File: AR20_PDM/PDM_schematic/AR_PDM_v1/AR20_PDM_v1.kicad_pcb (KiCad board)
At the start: 2 copper layers, 118 x 112 mm, 253 parts, among them IC1 TMUX1208PWR, J1 S_T_?, J2 1-776163-1, K1 DIPxx-1Cxx-51x, K2 DIPxx-1Cxx-51x, P1 B4B-PH-SM4-TB, Q1 BTS50025-1TAD, Q2 BTS50025-1TAD, Q3 BTS50025-1TAD, Q5 BTS50025-1TAD, Q6 BTS50025-1TAD, Q7 BTS50025-1TAD, Q8 BTS50025-1TAD, SW1 SW_DIP_x07, U1 ACM_2020, U10 N-MOS, U11 N-MOS, U12 P-MOS, U13 N-MOS, U14 N-MOS, U15 NMOS, U16 NMOS, U17 NMOS, U18 NMOS, U19 NMOS, U2 INA233, U20 NMOS, U21 NMOS, U22 NMOS, U23 NMOS, U24 NMOS, U25 NMOS, U26 NMOS, U27 NMOS, U28 NMOS, U29 INA233, U3 INA233, U30 INA233, U31 INA233, U32 Fet-P, U33 Fet-P, U34 Fet-P, U35 Fet-P, U36 Fet-P, U4 INA233, U5 INA233, U6 INA233, U7 INA233, U8 INA233, U9 TCA6424ARGJR

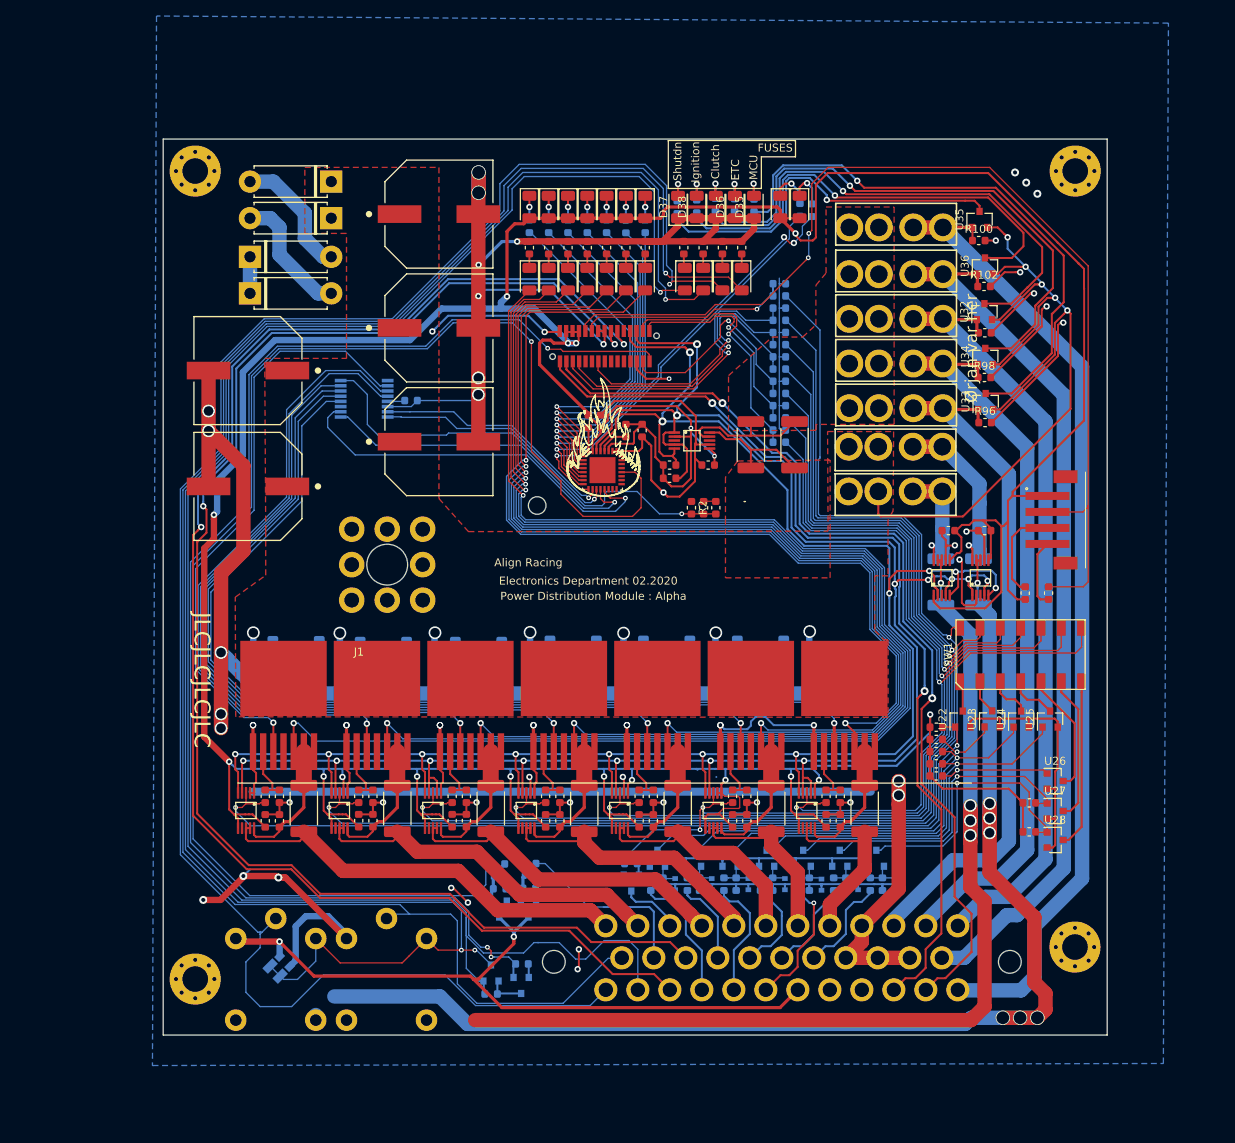
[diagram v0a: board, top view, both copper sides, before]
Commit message: Pdm version B Draft finished
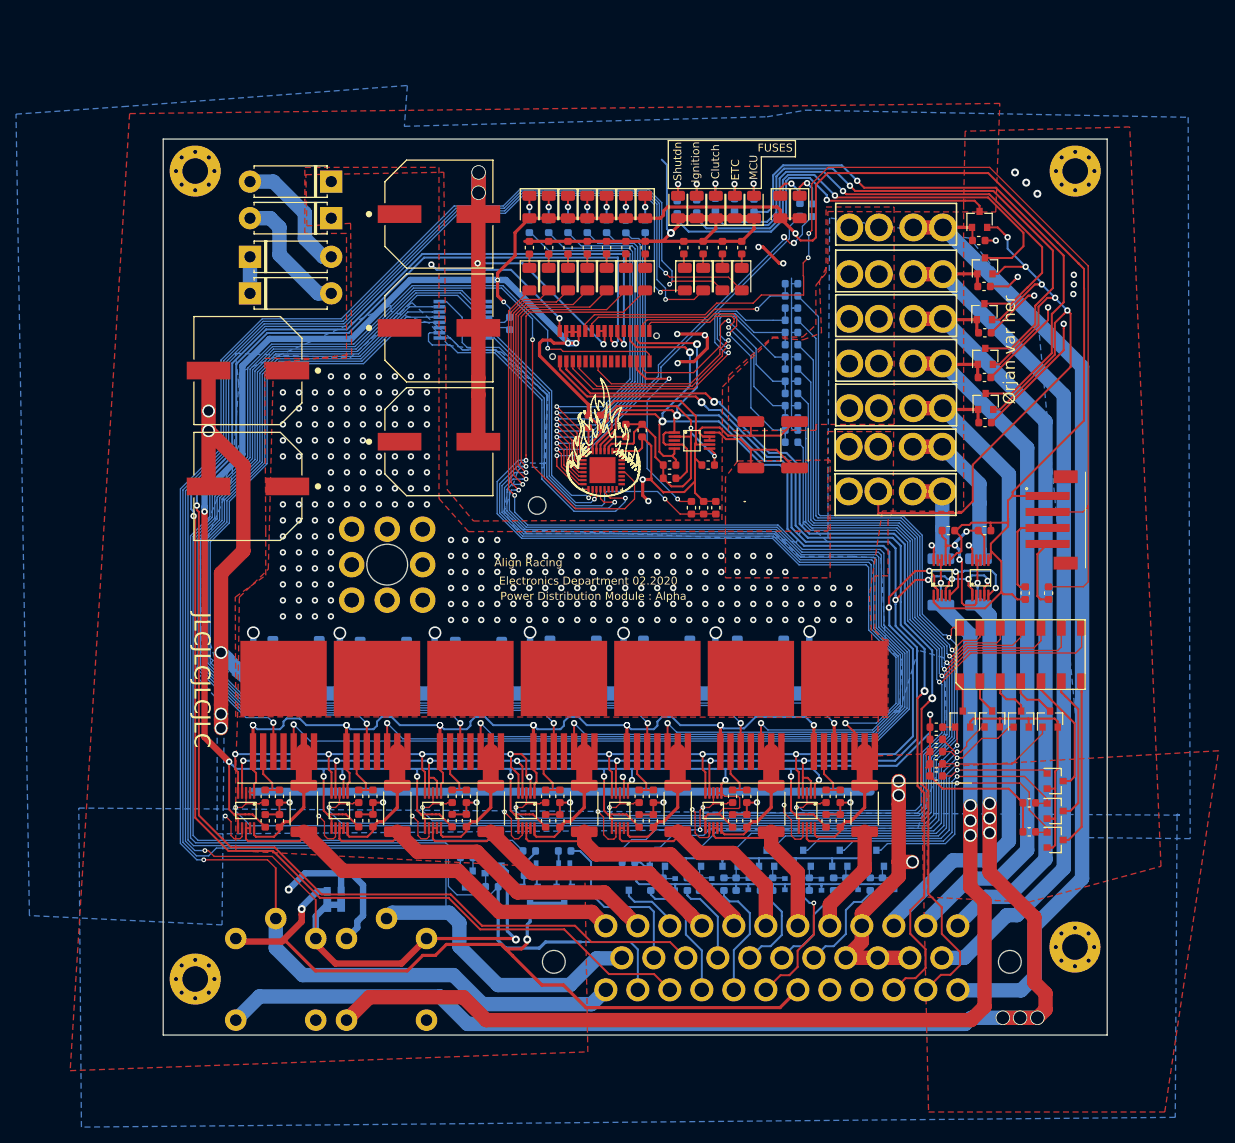
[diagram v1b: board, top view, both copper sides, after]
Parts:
- moved IC1 15.8 mm to (71.3, 58.9)
- moved C47 15.7 mm to (77.2, 59.4), turned to 270 degrees
- moved U11 15.0 mm to (71.6, 128.8)
- moved R89 15.0 mm to (71.8, 126.1)
- moved U12 13.4 mm to (75.1, 127.2), turned to 0 degrees
- moved R5 13.4 mm to (74.9, 129.8), turned to 0 degrees
- moved D30 11.6 mm to (56.1, 131.4), turned to 90 degrees
- moved D31 10.3 mm to (54.4, 131.4), turned to 90 degrees
- moved U14 4.79 mm to (84.0, 130.9)
- moved R92 4.66 mm to (84.0, 128.4)
- moved R105 4.64 mm to (84.0, 125.3)
- moved D40 4.61 mm to (84.0, 126.8)
- moved D39 4.30 mm to (79.8, 126.8)
- moved U13 4.23 mm to (79.7, 130.9)
- moved R90 4.21 mm to (79.8, 128.4)
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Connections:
- IC1 pad 3: (no net) -> Net-(IC1-Pad3)
- IC1 pad 9: (no net) -> Net-(IC1-Pad9)
- J2 pad 31: (no net) -> Net-(J2-Pad31)
- J2 pad 32: (no net) -> Net-(J2-Pad32)
- K1 pad 1: (no net) -> Net-(K1-Pad1)
- K2 pad 1: (no net) -> Net-(K2-Pad1)
- Q1 pad 4: (no net) -> Net-(Q1-Pad4)
- Q2 pad 4: (no net) -> Net-(Q2-Pad4)
- Q3 pad 4: (no net) -> Net-(Q3-Pad4)
- Q5 pad 4: (no net) -> Net-(Q5-Pad4)
- Q6 pad 4: (no net) -> Net-(Q6-Pad4)
- Q7 pad 4: (no net) -> Net-(Q7-Pad4)
- Q8 pad 4: (no net) -> Net-(Q8-Pad4)
- SW1 pad 12: (no net) -> P3_MOS_IN
- U1 pad 10: (no net) -> Net-(U1-Pad10)
- U1 pad 11: (no net) -> Net-(U1-Pad11)
- U1 pad 13: (no net) -> Net-(U1-Pad13)
- U1 pad 15: (no net) -> Net-(U1-Pad15)
- U1 pad 19: (no net) -> Net-(U1-Pad19)
- U1 pad 21: (no net) -> Net-(U1-Pad21)
- U1 pad 7: (no net) -> Net-(U1-Pad7)
- U1 pad 9: (no net) -> Net-(U1-Pad9)
- U29 pad 3: (no net) -> /Fuel_Ignition_ShutdownCircuit/COIL_INJECTOR_Alert
- U30 pad 3: (no net) -> /Fuel_Ignition_ShutdownCircuit/FP_Alert
- U31 pad 3: (no net) -> /Fuses_Direct/DIRECT_Alert
- U9 pad 14: (no net) -> Net-(U9-Pad14)
- U9 pad 15: (no net) -> Net-(U9-Pad15)
- U9 pad 16: (no net) -> Net-(U9-Pad16)
- U9 pad 17: (no net) -> Net-(U9-Pad17)
- U9 pad 18: (no net) -> Net-(U9-Pad18)
- U9 pad 19: (no net) -> Net-(U9-Pad19)
- U9 pad 21: (no net) -> Net-(U9-Pad21)
- U9 pad 22: (no net) -> Net-(U9-Pad22)
- U9 pad 23: (no net) -> Net-(U9-Pad23)
- U9 pad 24: (no net) -> Net-(U9-Pad24)
- U9 pad 33: (no net) -> Net-(U9-Pad33)
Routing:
- net GND: track 842.3 -> 961.9 mm, vias 56 -> 64
- net P7_MOS_SENSE: track 125.2 -> 147.7 mm
- net P6_MOS_SENSE: track 114.6 -> 137.0 mm
- net P5_MOS_SENSE: track 104.3 -> 126.5 mm
- net P4_MOS_SENSE: track 93.8 -> 115.7 mm
- net P3_MOS_SENSE: track 90.7 -> 112.4 mm
- net P2_MOS_SENSE: track 80.4 -> 101.4 mm
- net Net-(R2-Pad1): track 5.52 -> 25.1 mm, vias 1 -> 2
- net Net-(K1-Pad14): track 128.1 -> 146.6 mm
- net Shutdown_Relay_Side: track 228.1 -> 212.4 mm
- net P1_MOS_SENSE: track 75.5 -> 90.5 mm
- net FUEL_PUMP_OUT: track 227.8 -> 213.4 mm, vias 1 -> 2
- net Net-(K2-Pad14): track 159.8 -> 173.3 mm
- net TX: track 183.3 -> 192.8 mm
- net ACM_Shutdown_Circuit: track 168.1 -> 158.6 mm, vias 3 -> 1
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- added copper zone on F.Cu, net GND
- added copper zone on B.Cu, net V+12V
